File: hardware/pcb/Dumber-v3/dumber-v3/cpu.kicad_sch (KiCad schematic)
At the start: 27 parts, among them J1 Conn_02x03_Odd_Even, J2 Conn_02x03_Odd_Even, J3 Conn_02x05_Odd_Even, J4 TE 1-84982-0, M1 Motor, M2 Motor, Q2 PMN52XP, U1 XBEE-3, U2 STM32F071CBTx, U7 A3909

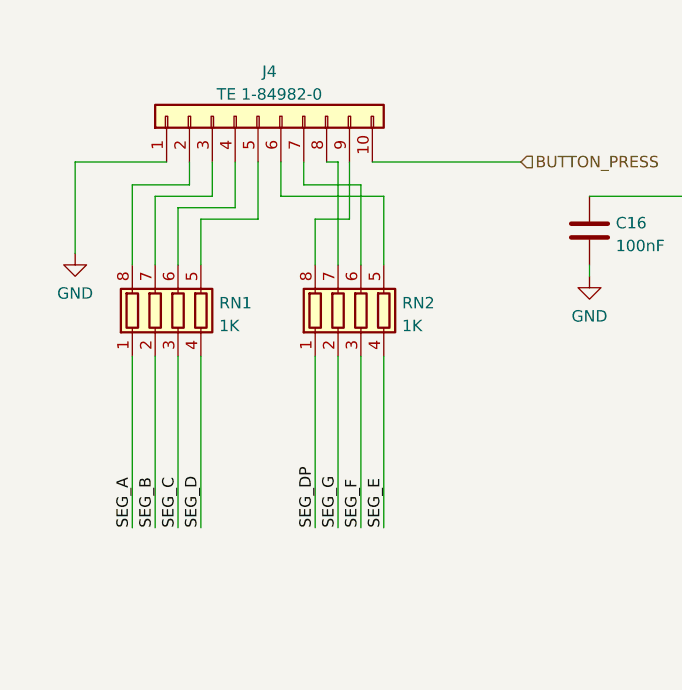
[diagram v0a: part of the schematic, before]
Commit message: Mise a jour sur les pcbs de dumber v3
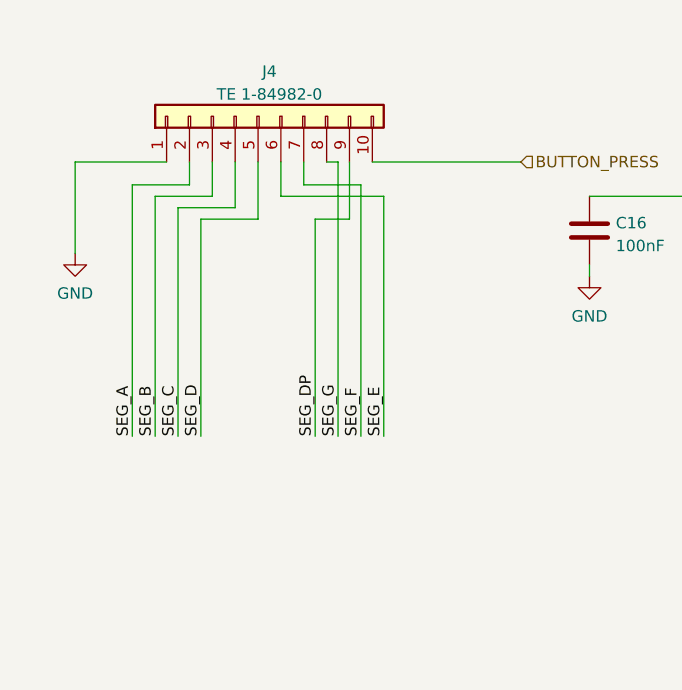
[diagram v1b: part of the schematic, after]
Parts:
- removed RN1, RN2: 1K, Resistor_SMD:R_Array_Convex_4x1206, symbol Device:R_Pack04
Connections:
- net SEG_A: now also J4.2 (Pin_2)
- net SEG_B: now also J4.3 (Pin_3)
- net SEG_C: now also J4.4 (Pin_4)
- net SEG_D: now also J4.5 (Pin_5)
- net SEG_DP: now also J4.9 (Pin_9)
- net SEG_E: now also J4.6 (Pin_6)
- net SEG_F: now also J4.7 (Pin_7)
- net SEG_G: now also J4.8 (Pin_8)
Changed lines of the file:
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@@
     (stroke (width 0) (type default) (color 0 0 0 0))
   )
-  (wire (pts (xy 39.37 50.8) (xy 39.37 45.72))
+  (wire (pts (xy 39.37 45.72) (xy 39.37 69.85))
     (stroke (width 0) (type default) (color 0 0 0 0))
   )
@@
     (stroke (width 0) (type default) (color 0 0 0 0))
   )
-  (wire (pts (xy 34.29 60.96) (xy 34.29 80.01))
-    (stroke (width 0) (type default) (color 0 0 0 0))
-  )
-  (wire (pts (xy 52.07 50.8) (xy 52.07 45.72))
+  (wire (pts (xy 52.07 45.72) (xy 52.07 69.85))
     (stroke (width 0) (type default) (color 0 0 0 0))
   )
@@
     (stroke (width 0) (type default) (color 0 0 0 0))
   )
-  (wire (pts (xy 36.83 50.8) (xy 36.83 44.45))
+  (wire (pts (xy 36.83 44.45) (xy 36.83 69.85))
     (stroke (width 0) (type default) (color 0 0 0 0))
   )
@@
     (stroke (width 0) (type default) (color 0 0 0 0))
   )
-  (wire (pts (xy 54.61 39.37) (xy 54.61 50.8))
+  (wire (pts (xy 54.61 39.37) (xy 54.61 69.85))
     (stroke (width 0) (type default) (color 0 0 0 0))
   )
@@
     (stroke (width 0) (type default) (color 0 0 0 0))
   )
-  (wire (pts (xy 31.75 60.96) (xy 31.75 80.01))
-    (stroke (width 0) (type default) (color 0 0 0 0))
-  )
   (wire (pts (xy 240.03 99.06) (xy 240.03 101.6))
     (stroke (width 0) (type default) (color 0 0 0 0))
@@
     (stroke (width 0) (type default) (color 0 0 0 0))
   )
-  (wire (pts (xy 54.61 60.96) (xy 54.61 80.01))
-    (stroke (width 0) (type default) (color 0 0 0 0))
-  )
   (wire (pts (xy 201.93 33.02) (xy 201.93 35.56))
     (stroke (width 0) (type default) (color 0 0 0 0))
   )
-  (wire (pts (xy 59.69 60.96) (xy 59.69 80.01))
-    (stroke (width 0) (type default) (color 0 0 0 0))
-  )
   (wire (pts (xy 232.41 29.21) (xy 232.41 38.1))
     (stroke (width 0) (type default) (color 0 0 0 0))
@@
     (stroke (width 0) (type default) (color 0 0 0 0))
   )
-  (wire (pts (xy 34.29 50.8) (xy 34.29 43.18))
+  (wire (pts (xy 34.29 43.18) (xy 34.29 69.85))
     (stroke (width 0) (type default) (color 0 0 0 0))
   )
@@
     (stroke (width 0) (type default) (color 0 0 0 0))
   )
-  (wire (pts (xy 57.15 50.8) (xy 57.15 41.91))
+  (wire (pts (xy 57.15 41.91) (xy 57.15 69.85))
     (stroke (width 0) (type default) (color 0 0 0 0))
   )
@@
     (stroke (width 0) (type default) (color 0 0 0 0))
   )
-  (wire (pts (xy 31.75 50.8) (xy 31.75 41.91))
-    (stroke (width 0) (type default) (color 0 0 0 0))
-  )
-  (wire (pts (xy 57.15 60.96) (xy 57.15 80.01))
+  (wire (pts (xy 31.75 41.91) (xy 31.75 69.85))
     (stroke (width 0) (type default) (color 0 0 0 0))
   )
@@
     (stroke (width 0) (type default) (color 0 0 0 0))
   )
-  (wire (pts (xy 59.69 50.8) (xy 59.69 43.18))
+  (wire (pts (xy 59.69 43.18) (xy 59.69 69.85))
     (stroke (width 0) (type default) (color 0 0 0 0))
   )
@@
     (stroke (width 0) (type default) (color 0 0 0 0))
   )
-  (wire (pts (xy 52.07 60.96) (xy 52.07 80.01))
-    (stroke (width 0) (type default) (color 0 0 0 0))
-  )
   (wire (pts (xy 110.49 78.74) (xy 116.84 78.74))
     (stroke (width 0) (type default) (color 0 0 0 0))
@@
     (stroke (width 0) (type default) (color 0 0 0 0))
   )
-  (wire (pts (xy 36.83 60.96) (xy 36.83 80.01))
-    (stroke (width 0) (type default) (color 0 0 0 0))
-  )
   (wire (pts (xy 113.03 48.26) (xy 116.84 48.26))
     (stroke (width 0) (type default) (color 0 0 0 0))
@@
     (stroke (width 0) (type default) (color 0 0 0 0))
   )
-  (wire (pts (xy 39.37 60.96) (xy 39.37 80.01))
-    (stroke (width 0) (type default) (color 0 0 0 0))
-  )
   (label "ENCDROIT_B" (at 172.72 78.74 180)
     (effects (font (size 1.27 1.27)) (justify right bottom))
@@
     (effects (font (size 1.27 1.27)) (justify right bottom))
   )
-  (label "SEG_F" (at 57.15 80.01 90)
-    (effects (font (size 1.27 1.27)) (justify left bottom))
-  )
-  (label "SEG_A" (at 31.75 80.01 90)
+  (label "SEG_F" (at 57.15 69.85 90)
+    (effects (font (size 1.27 1.27)) (justify left bottom))
+  )
+  (label "SEG_A" (at 31.75 69.85 90)
     (effects (font (size 1.27 1.27)) (justify left bottom))
   )
@@
     (effects (font (size 1.27 1.27)) (justify right bottom))
   )
-  (label "SEG_G" (at 54.61 80.01 90)
+  (label "SEG_G" (at 54.61 69.85 90)
     (effects (font (size 1.27 1.27)) (justify left bottom))
   )
@@
     (effects (font (size 1.27 1.27)) (justify right bottom))
   )
-  (label "SEG_C" (at 36.83 80.01 90)
-    (effects (font (size 1.27 1.27)) (justify left bottom))
-  )
-  (label "SEG_DP" (at 52.07 80.01 90)
+  (label "SEG_C" (at 36.83 69.85 90)
+    (effects (font (size 1.27 1.27)) (justify left bottom))
+  )
+  (label "SEG_DP" (at 52.07 69.85 90)
     (effects (font (size 1.27 1.27)) (justify left bottom))
   )
@@
     (effects (font (size 1.27 1.27)) (justify right bottom))
   )
-  (label "SEG_E" (at 59.69 80.01 90)
+  (label "SEG_E" (at 59.69 69.85 90)
     (effects (font (size 1.27 1.27)) (justify left bottom))
   )
@@
     (effects (font (size 1.27 1.27)) (justify right bottom))
   )
-  (label "SEG_B" (at 34.29 80.01 90)
+  (label "SEG_B" (at 34.29 69.85 90)
     (effects (font (size 1.27 1.27)) (justify left bottom))
   )
@@
     (effects (font (size 1.27 1.27)) (justify right bottom))
   )
-  (label "SEG_D" (at 39.37 80.01 90)
+  (label "SEG_D" (at 39.37 69.85 90)
     (effects (font (size 1.27 1.27)) (justify left bottom))
   )
@@
     (pin "1")
   )
-  (symbol (lib_id "Device:R_Pack04") (at 57.15 55.88 0) (unit 1)
-    (in_bom yes) (on_board yes) (fields_autoplaced)
-    (property "Reference" "RN2" (id 0) (at 61.722 55.0453 0)
-      (effects (font (size 1.27 1.27)) (justify left))
-    )
-    (property "Value" "1K" (id 1) (at 61.722 57.5822 0)
-      (effects (font (size 1.27 1.27)) (justify left))
-    )
-    (property "Footprint" "Resistor_SMD:R_Array_Convex_4x1206" (id 2) (at 64.135 55.88 90)
-      (effects (font (size 1.27 1.27)) hide)
-    )
-    (property "Datasheet" "~" (id 3) (at 57.15 55.88 0)
-      (effects (font (size 1.27 1.27)) hide)
-    )
-    (pin "1")
-    (pin "2")
-    (pin "3")
-    (pin "4")
-    (pin "5")
-    (pin "6")
-    (pin "7")
-    (pin "8")
-  )
   (symbol (lib_id "Device:C") (at 275.59 77.47 0) (unit 1)
     (in_bom yes) (on_board yes) (fields_autoplaced)
@@
     (pin "2")
   )
-  (symbol (lib_id "Device:R_Pack04") (at 36.83 55.88 0) (unit 1)
-    (in_bom yes) (on_board yes) (fields_autoplaced)
-    (property "Reference" "RN1" (id 0) (at 41.402 55.0453 0)
-      (effects (font (size 1.27 1.27)) (justify left))
-    )
-    (property "Value" "1K" (id 1) (at 41.402 57.5822 0)
-      (effects (font (size 1.27 1.27)) (justify left))
-    )
-    (property "Footprint" "Resistor_SMD:R_Array_Convex_4x1206" (id 2) (at 43.815 55.88 90)
-      (effects (font (size 1.27 1.27)) hide)
-    )
-    (property "Datasheet" "~" (id 3) (at 36.83 55.88 0)
-      (effects (font (size 1.27 1.27)) hide)
-    )
-    (pin "1")
-    (pin "2")
-    (pin "3")
-    (pin "4")
-    (pin "5")
-    (pin "6")
-    (pin "7")
-    (pin "8")
-  )
   (symbol (lib_id "power:GND") (at 49.53 175.26 0) (unit 1)
